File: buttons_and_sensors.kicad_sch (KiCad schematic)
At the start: 11 parts, among them CN13 4P JST ZH, CN14 4P JST ZH, CN5 4P JST ZH

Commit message: Updated library name, updated and verified all footprints
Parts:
- C22: footprint easyeda2kicad:C0805 -> LiveAstra:C0805; symbol EASYEDA2KICAD:C_100pF_C0G_0805 -> LiveAstra:C_100pF_C0G_0805
- CN13, CN14, CN5: footprint EASYEDA2KICAD:CONN-TH_B4B-ZR-3.4-LF-SN -> LiveAstra:CONN-TH_B4B-ZR-3.4-LF-SN; symbol EASYEDA2KICAD:JST_ZH_4PIN_1A_50V -> LiveAstra:JST_ZH_4PIN_1A_50V
- R1, R2, R22, R29: footprint EASYEDA2KICAD:R0402 -> LiveAstra:R0402; symbol EASYEDA2KICAD:R_5k1_0402_62mW -> LiveAstra:R_5k1_0402_62mW
- R23: footprint EASYEDA2KICAD:R0402 -> LiveAstra:R0402; symbol EASYEDA2KICAD:R_10kOhm_0402_62mW -> LiveAstra:R_10kOhm_0402_62mW
- R28: footprint easyeda2kicad:R0805 -> LiveAstra:R0805; symbol EASYEDA2KICAD:R_3k3Ohm_0805_125mW -> LiveAstra:R_3k3Ohm_0805_125mW
- R30: footprint EASYEDA2KICAD:R0805 -> LiveAstra:R0805; symbol EASYEDA2KICAD:R_0Ohm_0805_125mW -> LiveAstra:R_0Ohm_0805_125mW
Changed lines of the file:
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@@
 	)
 	(symbol
-		(lib_id "EASYEDA2KICAD:JST_ZH_4PIN_1A_50V")
+		(lib_id "LiveAstra:JST_ZH_4PIN_1A_50V")
 		(at 106.68 50.8 180)
 		(unit 1)
@@
 			)
 		)
-		(property "Footprint" "EASYEDA2KICAD:CONN-TH_B4B-ZR-3.4-LF-SN"
+		(property "Footprint" "LiveAstra:CONN-TH_B4B-ZR-3.4-LF-SN"
 			(at 106.68 34.29 0)
 			(effects
@@
 	)
 	(symbol
-		(lib_id "EASYEDA2KICAD:JST_ZH_4PIN_1A_50V")
+		(lib_id "LiveAstra:JST_ZH_4PIN_1A_50V")
 		(at 106.68 152.4 180)
 		(unit 1)
@@
 			)
 		)
-		(property "Footprint" "EASYEDA2KICAD:CONN-TH_B4B-ZR-3.4-LF-SN"
+		(property "Footprint" "LiveAstra:CONN-TH_B4B-ZR-3.4-LF-SN"
 			(at 106.68 135.89 0)
 			(effects
@@
 	)
 	(symbol
-		(lib_id "EASYEDA2KICAD:R_5k1_0402_62mW")
+		(lib_id "LiveAstra:R_5k1_0402_62mW")
 		(at 124.46 86.36 90)
 		(unit 1)
@@
 			)
 		)
-		(property "Footprint" "EASYEDA2KICAD:R0402"
+		(property "Footprint" "LiveAstra:R0402"
 			(at 133.35 86.36 0)
 			(effects
@@
 	)
 	(symbol
-		(lib_id "EASYEDA2KICAD:R_5k1_0402_62mW")
+		(lib_id "LiveAstra:R_5k1_0402_62mW")
 		(at 177.8 91.44 90)
 		(unit 1)
@@
 			)
 		)
-		(property "Footprint" "EASYEDA2KICAD:R0402"
+		(property "Footprint" "LiveAstra:R0402"
 			(at 186.69 91.44 0)
 			(effects
@@
 	)
 	(symbol
-		(lib_id "EASYEDA2KICAD:C_100pF_C0G_0805")
+		(lib_id "LiveAstra:C_100pF_C0G_0805")
 		(at 203.2 55.88 90)
 		(unit 1)
@@
 			)
 		)
-		(property "Footprint" "easyeda2kicad:C0805"
+		(property "Footprint" "LiveAstra:C0805"
 			(at 215.9 55.88 0)
 			(effects
@@
 	)
 	(symbol
-		(lib_id "EASYEDA2KICAD:R_10kOhm_0402_62mW")
+		(lib_id "LiveAstra:R_10kOhm_0402_62mW")
 		(at 152.4 40.64 90)
 		(unit 1)
@@
 			)
 		)
-		(property "Footprint" "EASYEDA2KICAD:R0402"
+		(property "Footprint" "LiveAstra:R0402"
 			(at 165.1 40.64 0)
 			(effects
@@
 	)
 	(symbol
-		(lib_id "EASYEDA2KICAD:R_5k1_0402_62mW")
+		(lib_id "LiveAstra:R_5k1_0402_62mW")
 		(at 177.8 142.24 90)
 		(unit 1)
@@
 			)
 		)
-		(property "Footprint" "EASYEDA2KICAD:R0402"
+		(property "Footprint" "LiveAstra:R0402"
 			(at 186.69 142.24 0)
 			(effects
@@
 	)
 	(symbol
-		(lib_id "EASYEDA2KICAD:R_5k1_0402_62mW")
+		(lib_id "LiveAstra:R_5k1_0402_62mW")
 		(at 124.46 137.16 90)
 		(unit 1)
@@
 			)
 		)
-		(property "Footprint" "EASYEDA2KICAD:R0402"
+		(property "Footprint" "LiveAstra:R0402"
 			(at 133.35 137.16 0)
 			(effects
@@
 	)
 	(symbol
-		(lib_id "EASYEDA2KICAD:R_3k3Ohm_0805_125mW")
+		(lib_id "LiveAstra:R_3k3Ohm_0805_125mW")
 		(at 193.04 48.26 0)
 		(unit 1)
@@
 			)
 		)
-		(property "Footprint" "easyeda2kicad:R0805"
+		(property "Footprint" "LiveAstra:R0805"
 			(at 193.04 57.15 0)
 			(effects
@@
 	)
 	(symbol
-		(lib_id "EASYEDA2KICAD:R_0Ohm_0805_125mW")
+		(lib_id "LiveAstra:R_0Ohm_0805_125mW")
 		(at 121.92 43.18 0)
 		(unit 1)
@@
 			)
 		)
-		(property "Footprint" "EASYEDA2KICAD:R0805"
+		(property "Footprint" "LiveAstra:R0805"
 			(at 121.92 55.88 0)
 			(effects
@@
 	)
 	(symbol
-		(lib_id "EASYEDA2KICAD:JST_ZH_4PIN_1A_50V")
+		(lib_id "LiveAstra:JST_ZH_4PIN_1A_50V")
 		(at 106.68 101.6 180)
 		(unit 1)
@@
 			)
 		)
-		(property "Footprint" "EASYEDA2KICAD:CONN-TH_B4B-ZR-3.4-LF-SN"
+		(property "Footprint" "LiveAstra:CONN-TH_B4B-ZR-3.4-LF-SN"
 			(at 106.68 85.09 0)
 			(effects

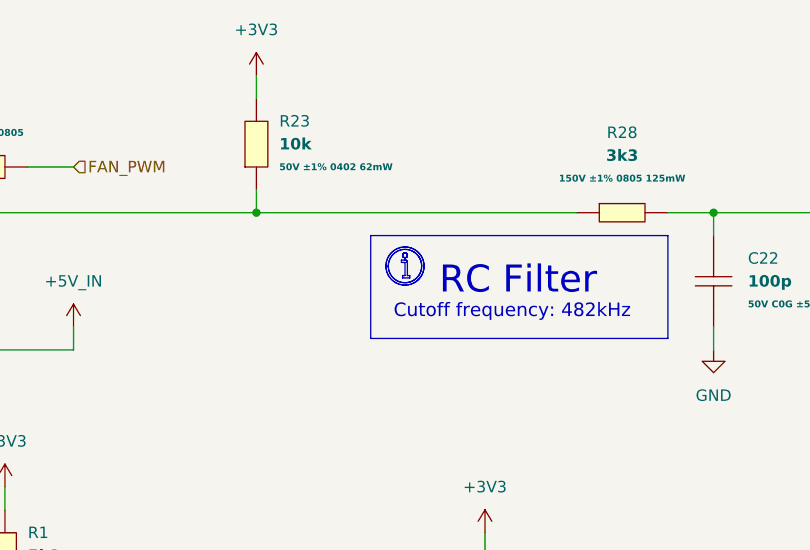
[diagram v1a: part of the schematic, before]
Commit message: Work on kibot
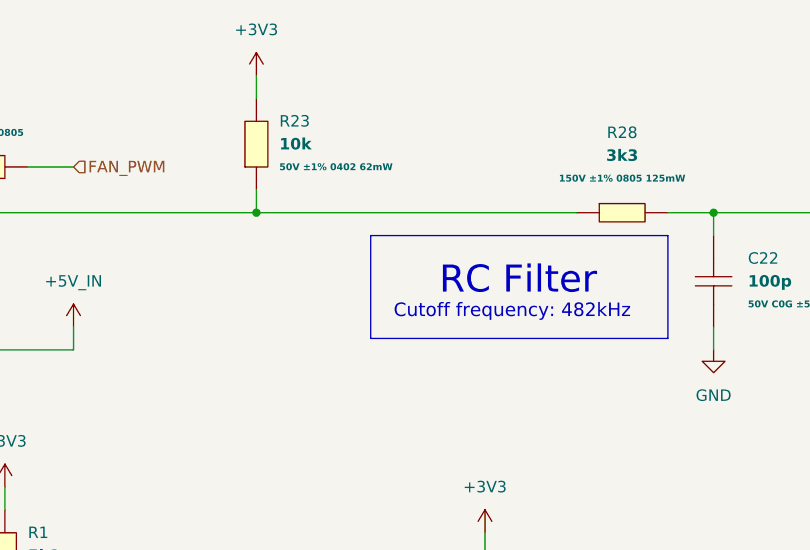
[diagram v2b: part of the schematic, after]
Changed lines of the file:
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@@
-		)
-	)
-	(polyline
-		(pts
-			(xy 168.9236 52.7318) (xy 168.937 52.7328) (xy 168.9503 52.7345) (xy 168.9633 52.7368) (xy 168.9761 52.7398)
-			(xy 168.9886 52.7434) (xy 169.0009 52.7475) (xy 169.013 52.7523) (xy 169.0247 52.7575) (xy 169.0361 52.7634)
-			(xy 169.0472 52.7698) (xy 169.0579 52.7766) (xy 169.0683 52.784) (xy 169.0783 52.7919) (xy 169.0879 52.8002)
-			(xy 169.0971 52.809) (xy 169.1058 52.8181) (xy 169.1141 52.8277) (xy 169.122 52.8377) (xy 169.1294 52.8481)
-			(xy 169.1362 52.8588) (xy 169.1426 52.8699) (xy 169.1485 52.8813) (xy 169.1538 52.8931) (xy 169.1585 52.9051)
-			(xy 169.1627 52.9174) (xy 169.1662 52.9299) (xy 169.1692 52.9427) (xy 169.1715 52.9557) (xy 169.1732 52.969)
-			(xy 169.1742 52.9824) (xy 169.1745 52.996) (xy 169.1742 53.0097) (xy 169.1732 53.0231) (xy 169.1715 53.0363)
-			(xy 169.1692 53.0494) (xy 169.1662 53.0622) (xy 169.1627 53.0747) (xy 169.1585 53.087) (xy 169.1538 53.099)
-			(xy 169.1485 53.1107) (xy 169.1426 53.1222) (xy 169.1362 53.1332) (xy 169.1294 53.144) (xy 169.122 53.1543)
-			(xy 169.1141 53.1643) (xy 169.1058 53.1739) (xy 169.0971 53.1831) (xy 169.0879 53.1919) (xy 169.0783 53.2002)
-			(xy 169.0683 53.2081) (xy 169.0579 53.2154) (xy 169.0472 53.2223) (xy 169.0361 53.2287) (xy 169.0247 53.2345)
-			(xy 169.013 53.2398) (xy 169.0009 53.2446) (xy 168.9886 53.2487) (xy 168.9761 53.2523) (xy 168.9633 53.2552)
-			(xy 168.9503 53.2576) (xy 168.937 53.2593) (xy 168.9236 53.2603) (xy 168.91 53.2606) (xy 168.8964 53.2603)
-			(xy 168.8829 53.2593) (xy 168.8697 53.2576) (xy 168.8566 53.2552) (xy 168.8438 53.2523) (xy 168.8313 53.2487)
-			(xy 168.819 53.2446) (xy 168.807 53.2398) (xy 168.7953 53.2345) (xy 168.7839 53.2287) (xy 168.7728 53.2223)
-			(xy 168.762 53.2154) (xy 168.7517 53.2081) (xy 168.7417 53.2002) (xy 168.7321 53.1919) (xy 168.7229 53.1831)
-			(xy 168.7141 53.1739) (xy 168.7058 53.1643) (xy 168.6979 53.1543) (xy 168.6906 53.144) (xy 168.6837 53.1332)
-			(xy 168.6773 53.1222) (xy 168.6715 53.1107) (xy 168.6662 53.099) (xy 168.6614 53.087) (xy 168.6573 53.0747)
-			(xy 168.6537 53.0622) (xy 168.6508 53.0494) (xy 168.6484 53.0363) (xy 168.6467 53.0231) (xy 168.6457 53.0097)
-			(xy 168.6454 52.996) (xy 168.6457 52.9824) (xy 168.6467 52.969) (xy 168.6484 52.9557) (xy 168.6508 52.9427)
-			(xy 168.6537 52.9299) (xy 168.6573 52.9174) (xy 168.6614 52.9051) (xy 168.6662 52.8931) (xy 168.6715 52.8813)
-			(xy 168.6773 52.8699) (xy 168.6837 52.8588) (xy 168.6906 52.8481) (xy 168.6979 52.8377) (xy 168.7058 52.8277)
-			(xy 168.7141 52.8181) (xy 168.7229 52.809) (xy 168.7321 52.8002) (xy 168.7417 52.7919) (xy 168.7517 52.784)
-			(xy 168.762 52.7766) (xy 168.7728 52.7698) (xy 168.7839 52.7634) (xy 168.7953 52.7575) (xy 168.807 52.7523)
-			(xy 168.819 52.7475) (xy 168.8313 52.7434) (xy 168.8438 52.7398) (xy 168.8566 52.7368) (xy 168.8697 52.7345)
-			(xy 168.8829 52.7328) (xy 168.8964 52.7318) (xy 168.91 52.7315) (xy 168.9236 52.7318)
-		)
-		(stroke
-			(width -0.0001)
-			(type solid)
-		)
-		(fill
-			(type color)
-			(color 34 187 51 1)
-		)
-	)
-	(polyline
-		(pts
-			(xy 168.9231 53.5255) (xy 168.9361 53.5265) (xy 168.949 53.5281) (xy 168.9618 53.5303) (xy 168.9745 53.5332)
-			(xy 168.9869 53.5366) (xy 168.9992 53.5407) (xy 169.0112 53.5453) (xy 169.023 53.5506) (xy 169.0346 53.5564)
-			(xy 169.0458 53.5627) (xy 169.0568 53.5697) (xy 169.0674 53.5771) (xy 169.0776 53.5851) (xy 169.0875 53.5937)
-			(xy 169.0971 53.6027) (xy 169.1061 53.6122) (xy 169.1146 53.6221) (xy 169.1226 53.6324) (xy 169.1301 53.643)
-			(xy 169.137 53.6539) (xy 169.1434 53.6652) (xy 169.1492 53.6767) (xy 169.1544 53.6885) (xy 169.1591 53.7006)
-			(xy 169.1631 53.7128) (xy 169.1666 53.7253) (xy 169.1694 53.7379) (xy 169.1717 53.7507) (xy 169.1733 53.7636)
-			(xy 169.1742 53.7767) (xy 169.1745 53.7898) (xy 169.1745 55.245) (xy 169.4391 55.245) (xy 169.4391 55.5096)
-			(xy 168.6454 55.5096) (xy 168.6454 55.245) (xy 168.91 55.245) (xy 168.91 53.7898) (xy 168.5131 53.7898)
-			(xy 168.5131 53.5252) (xy 168.91 53.5252) (xy 168.9231 53.5255)
-		)
-		(stroke
-			(width -0.0001)
-			(type solid)
-		)
-		(fill
-			(type color)
-			(color 34 187 51 1)
-		)
-	)
-	(polyline
-		(pts
-			(xy 169.0149 52.0726) (xy 169.1192 52.0804) (xy 169.2225 52.0932) (xy 169.3248 52.111) (xy 169.4259 52.1338)
-			(xy 169.5256 52.1615) (xy 169.6237 52.1939) (xy 169.72 52.2311) (xy 169.8144 52.2729) (xy 169.9067 52.3194)
-			(xy 169.9967 52.3703) (xy 170.0843 52.4256) (xy 170.1693 52.4853) (xy 170.2514 52.5493) (xy 170.3306 52.6176)
-			(xy 170.4067 52.69) (xy 170.4791 52.766) (xy 170.5473 52.8452) (xy 170.6113 52.9274) (xy 170.671 53.0123)
-			(xy 170.7264 53.0999) (xy 170.7773 53.1899) (xy 170.8237 53.2823) (xy 170.8655 53.3767) (xy 170.9027 53.473)
-			(xy 170.9351 53.5711) (xy 170.9628 53.6707) (xy 170.9856 53.7718) (xy 171.0034 53.8741) (xy 171.0163 53.9775)
-			(xy 171.024 54.0817) (xy 171.0266 54.1867) (xy 171.0251 54.2667) (xy 171.0206 54.3461) (xy 171.0132 54.4249)
-			(xy 171.0029 54.5031) (xy 170.9898 54.5804) (xy 170.9738 54.657) (xy 170.9551 54.7326) (xy 170.9337 54.8073)
-			(xy 170.9096 54.881) (xy 170.8829 54.9536) (xy 170.8536 55.025) (xy 170.8217 55.0952) (xy 170.7874 55.1642)
-			(xy 170.7506 55.2318) (xy 170.7115 55.2979) (xy 170.6699 55.3626) (xy 170.626 55.4258) (xy 170.5799 55.4873)
-			(xy 170.5315 55.5471) (xy 170.481 55.6052) (xy 170.4283 55.6615) (xy 170.3735 55.7159) (xy 170.3167 55.7684)
-			(xy 170.2578 55.8188) (xy 170.197 55.8672) (xy 170.1343 55.9134) (xy 170.0697 55.9575) (xy 170.0032 55.9992)
-			(xy 169.935 56.0387) (xy 169.865 56.0757) (xy 169.7933 56.1102) (xy 169.72 56.1422) (xy 169.5704 56.1977)
-			(xy 169.4186 56.2414) (xy 169.2653 56.2734) (xy 169.111 56.2939) (xy 168.9564 56.3029) (xy 168.8022 56.3006)
-			(xy 168.6488 56.2872) (xy 168.497 56.2627) (xy 168.3474 56.2272) (xy 168.2006 56.181) (xy 168.0572 56.124)
-			(xy 167.9178 56.0565) (xy 167.7831 55.9786) (xy 167.6537 55.8903) (xy 167.5302 55.7919) (xy 167.4133 55.6834)
-			(xy 167.3047 55.5664) (xy 167.2063 55.4429) (xy 167.118 55.3135) (xy 167.0401 55.1788) (xy 166.9726 55.0394)
-			(xy 166.9157 54.896) (xy 166.8694 54.7492) (xy 166.834 54.5996) (xy 166.8095 54.4478) (xy 166.796 54.2945)
-			(xy 166.795 54.2273) (xy 167.0583 54.2273) (xy 167.0662 54.3626) (xy 167.0841 54.4976) (xy 167.1121 54.6317)
-			(xy 167.1503 54.7645) (xy 167.1989 54.8954) (xy 167.2571 55.0223) (xy 167.324 55.1433) (xy 167.399 55.2579)
-			(xy 167.4818 55.366) (xy 167.5719 55.4673) (xy 167.6687 55.5613) (xy 167.7719 55.6479) (xy 167.881 55.7266)
-			(xy 167.9955 55.7973) (xy 168.115 55.8595) (xy 168.2389 55.913) (xy 168.3669 55.9574) (xy 168.4985 55.9925)
-			(xy 168.6331 56.018) (xy 168.7705 56.0335) (xy 168.91 56.0387) (xy 169.0018 56.0365) (xy 169.093 56.0297)
-			(xy 169.1835 56.0185) (xy 169.273 56.0028) (xy 169.3614 55.9829) (xy 169.4486 55.9587) (xy 169.5344 55.9303)
-			(xy 169.6187 55.8978) (xy 169.7013 55.8612) (xy 169.7821 55.8206) (xy 169.8609 55.776) (xy 169.9375 55.7276)
-			(xy 170.0118 55.6753) (xy 170.0837 55.6193) (xy 170.153 55.5596) (xy 170.2196 55.4963) (xy 170.2829 55.4297)
-			(xy 170.3426 55.3604) (xy 170.3986 55.2885) (xy 170.4509 55.2142) (xy 170.4993 55.1376) (xy 170.5439 55.0588)
-			(xy 170.5845 54.978) (xy 170.6211 54.8954) (xy 170.6536 54.8111) (xy 170.682 54.7253) (xy 170.7062 54.6381)
-			(xy 170.7261 54.5497) (xy 170.7418 54.4602) (xy 170.753 54.3697) (xy 170.7598 54.2785) (xy 170.762 54.1867)
-			(xy 170.7607 54.1167) (xy 170.7568 54.0472) (xy 170.7503 53.9782) (xy 170.7413 53.9098) (xy 170.7298 53.8421)
-			(xy 170.7158 53.7752) (xy 170.6995 53.709) (xy 170.6807 53.6436) (xy 170.6596 53.5791) (xy 170.6363 53.5156)
-			(xy 170.6106 53.4531) (xy 170.5828 53.3917) (xy 170.5527 53.3313) (xy 170.5206 53.2722) (xy 170.4863 53.2143)
-			(xy 170.4499 53.1577) (xy 170.4115 53.1025) (xy 170.3712 53.0486) (xy 170.3288 52.9963) (xy 170.2846 52.9454)
-			(xy 170.2385 52.8962) (xy 170.1906 52.8486) (xy 170.1408 52.8027) (xy 170.0893 52.7585) (xy 170.0361 52.7162)
-			(xy 169.9812 52.6757) (xy 169.9247 52.6372) (xy 169.8666 52.6007) (xy 169.8069 52.5662) (xy 169.7456 52.5338)
-			(xy 169.6829 52.5036) (xy 169.6187 52.4756) (xy 169.4878 52.427) (xy 169.355 52.3888) (xy 169.2209 52.3608)
-			(xy 169.0859 52.3429) (xy 168.9506 52.335) (xy 168.8156 52.337) (xy 168.6815 52.3487) (xy 168.5486 52.3702)
-			(xy 168.4177 52.4012) (xy 168.2893 52.4417) (xy 168.1638 52.4915) (xy 168.0419 52.5505) (xy 167.924 52.6187)
-			(xy 167.8108 52.696) (xy 167.7027 52.7821) (xy 167.6003 52.877) (xy 167.5054 52.9794) (xy 167.4193 53.0875)
-			(xy 167.342 53.2007) (xy 167.2738 53.3186) (xy 167.2148 53.4405) (xy 167.165 53.566) (xy 167.1245 53.6944)
-			(xy 167.0935 53.8253) (xy 167.072 53.9582) (xy 167.0603 54.0923) (xy 167.0583 54.2273) (xy 166.795 54.2273)
-			(xy 166.7937 54.1402) (xy 166.8028 53.9856) (xy 166.8232 53.8314) (xy 166.8552 53.678) (xy 166.8989 53.5263)
-			(xy 166.9544 53.3767) (xy 167.021 53.2316) (xy 167.0974 53.0934) (xy 167.1832 52.9624) (xy 167.2778 52.8388)
-			(xy 167.3807 52.7231) (xy 167.4914 52.6156) (xy 167.6093 52.5167) (xy 167.734 52.4267) (xy 167.8649 52.346)
-			(xy 168.0014 52.2749) (xy 168.143 52.2137) (xy 168.2893 52.1629) (xy 168.4397 52.1228) (xy 168.5936 52.0937)
-			(xy 168.7505 52.076) (xy 168.91 52.07) (xy 169.0149 52.0726)
-		)
-		(stroke
-			(width -0.0001)
-			(type solid)
-		)
-		(fill
-			(type color)
-			(color 34 187 51 1)
 		)
 	)
